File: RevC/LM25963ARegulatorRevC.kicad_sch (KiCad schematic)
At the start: 11 parts, among them J1 Screw_Terminal_01x02, J2 Screw_Terminal_01x02, U1 LM2596S-ADJ

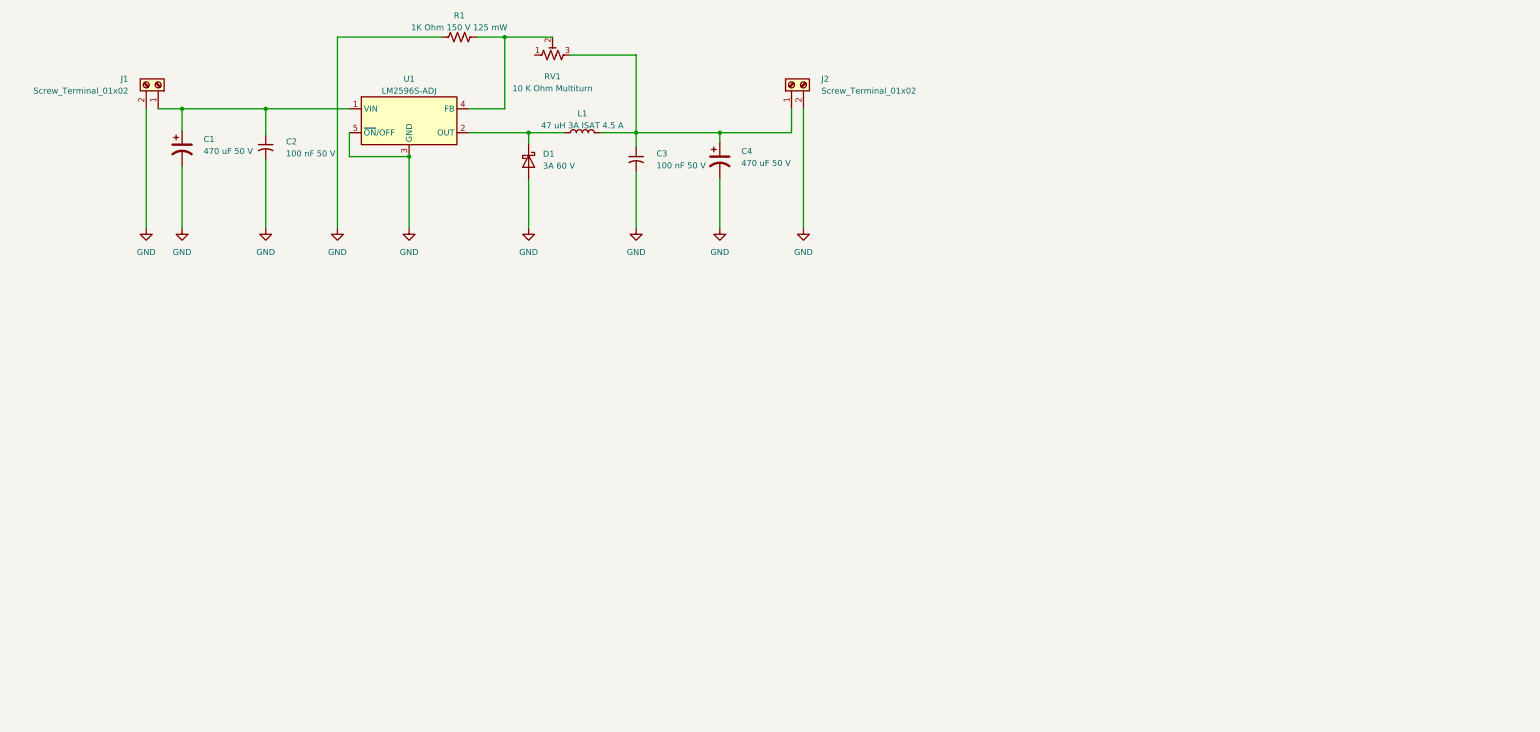
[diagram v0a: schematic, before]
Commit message: Add files via upload
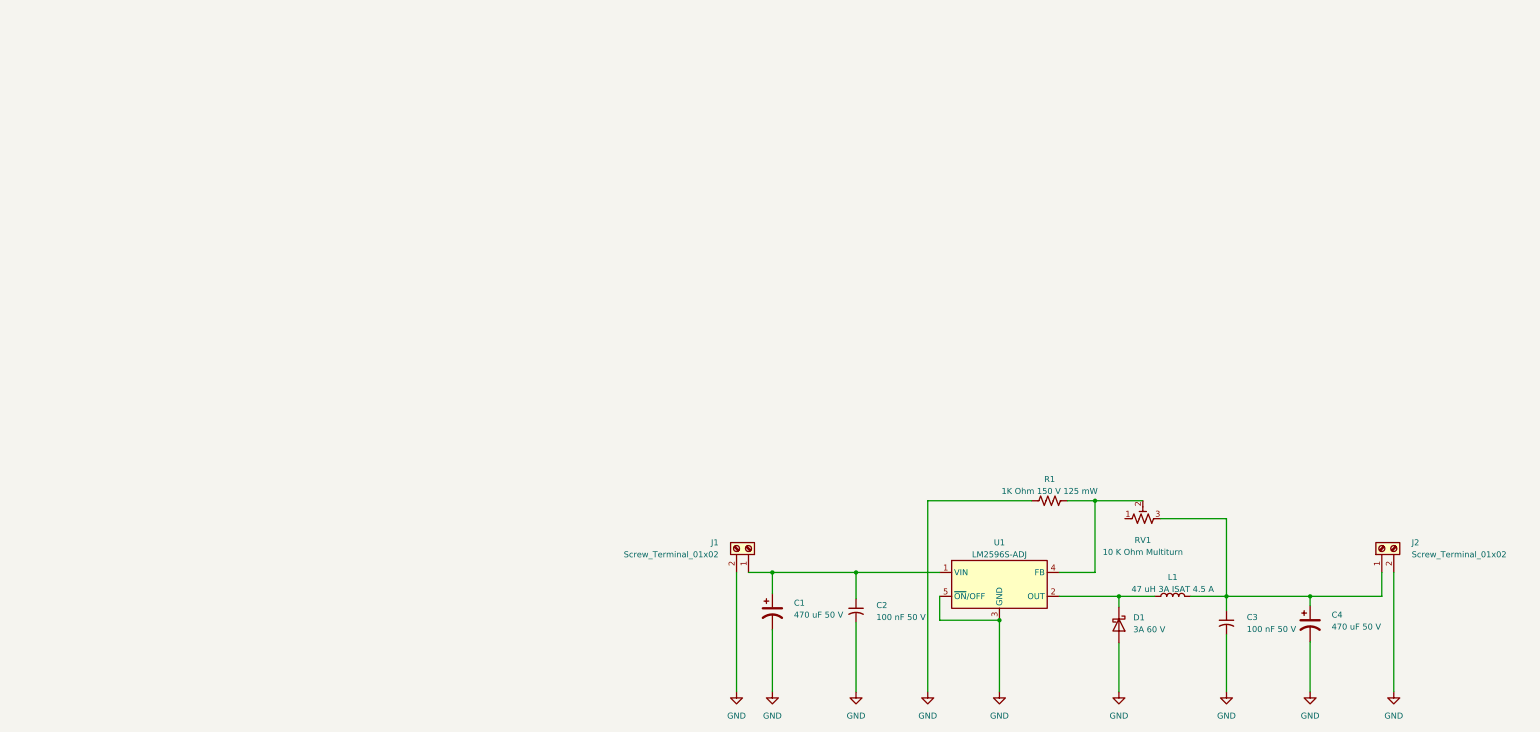
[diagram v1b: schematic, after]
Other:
- company: (none) -> Yasa Teknoloji
- title: (none) -> LM2596 3A Regulator Project
- moved on the sheet: C1, C2, C3, C4, D1, J1, J2, L1, R1, RV1, U1
